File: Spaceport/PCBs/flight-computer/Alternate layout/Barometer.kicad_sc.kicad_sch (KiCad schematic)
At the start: 2 parts, among them U1 MS5611-01BA

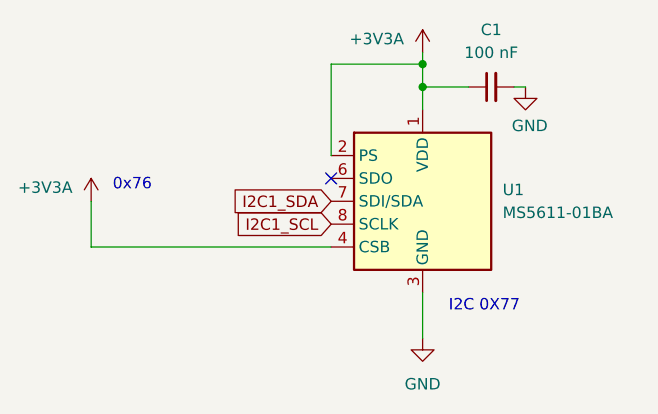
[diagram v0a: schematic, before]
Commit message: removed all global labels
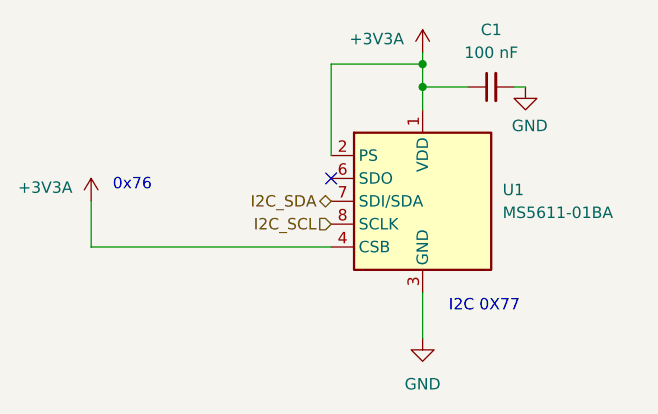
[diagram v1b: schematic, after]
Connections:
- net I2C1_SCL renamed I2C_SCL
- net I2C1_SDA renamed I2C_SDA
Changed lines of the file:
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@@
 		)
 	)
-	(global_label "I2C1_SDA"
+	(hierarchical_label "I2C_SCL"
 		(shape input)
-		(at 116.84 71.12 180)
-		(fields_autoplaced yes)
+		(at 116.84 73.66 180)
 		(effects
 			(font
@@
 			(justify right)
 		)
-		(property "Intersheetrefs" "${INTERSHEET_REFS}"
-			(at 105.0253 71.12 0)
-			(effects
-				(font
-					(size 1.27 1.27)
-				)
-				(justify right)
-				(hide yes)
-			)
-		)
 	)
-	(global_label "I2C1_SCL"
-		(shape input)
-		(at 116.84 73.66 180)
-		(fields_autoplaced yes)
+	(hierarchical_label "I2C_SDA"
+		(shape bidirectional)
+		(at 116.84 71.12 180)
 		(effects
 			(font
@@
 			(justify right)
 		)
-		(property "Intersheetrefs" "${INTERSHEET_REFS}"
-			(at 105.0858 73.66 0)
-			(effects
-				(font
-					(size 1.27 1.27)
-				)
-				(justify right)
-				(hide yes)
-			)
-		)
 	)
